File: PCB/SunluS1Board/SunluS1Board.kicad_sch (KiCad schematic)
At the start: 19 parts, among them M1 Fan, Q1 AO3400A, Q2 AO3400A, SW1 CS1213AGF260, SW2 CS1213AGF260, U1 STM32C011F4Px

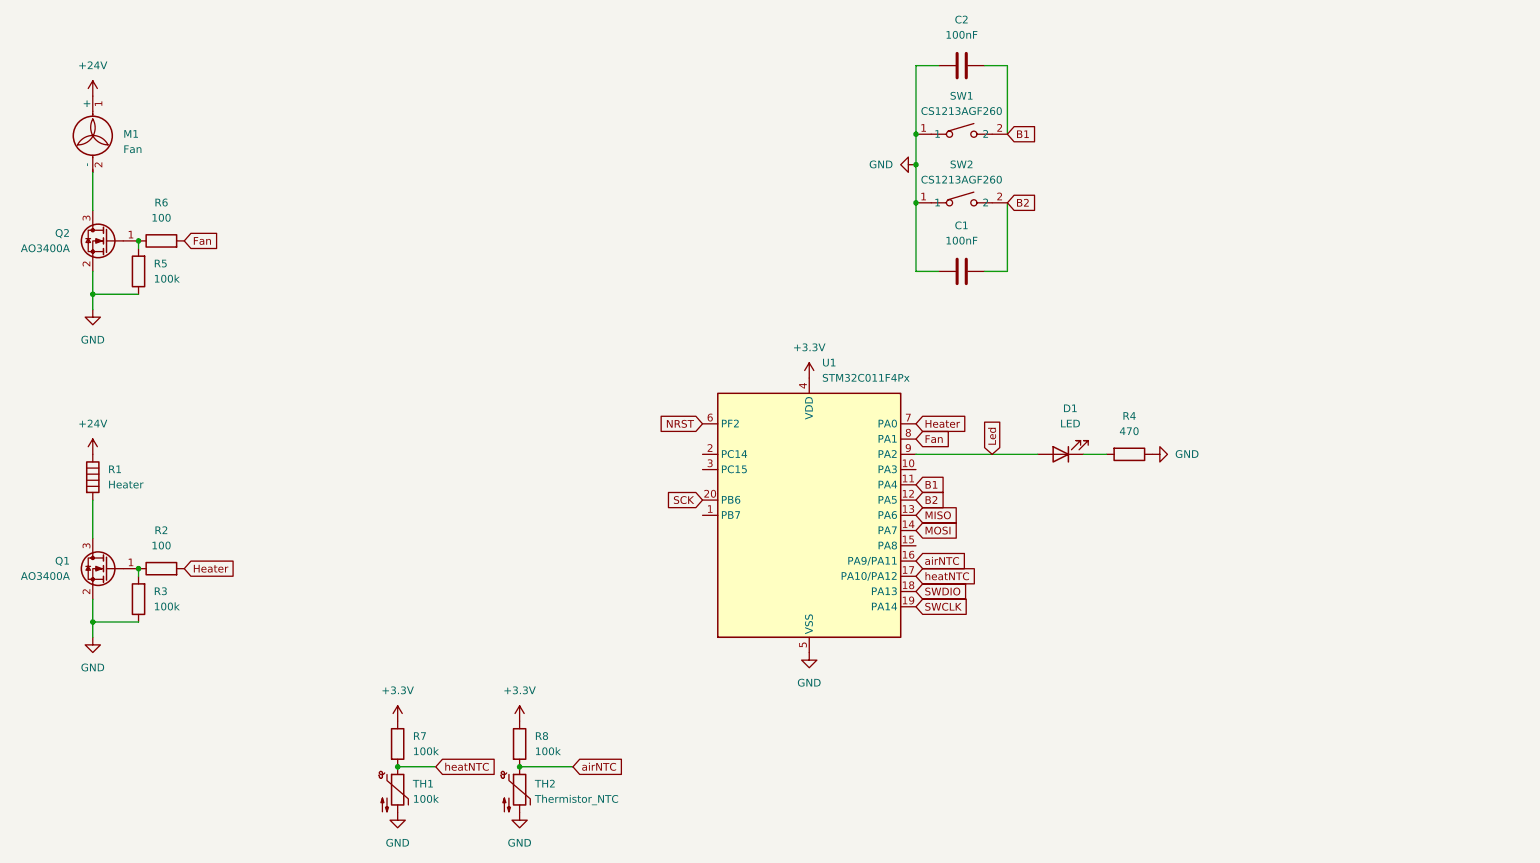
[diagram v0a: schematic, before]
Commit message: display
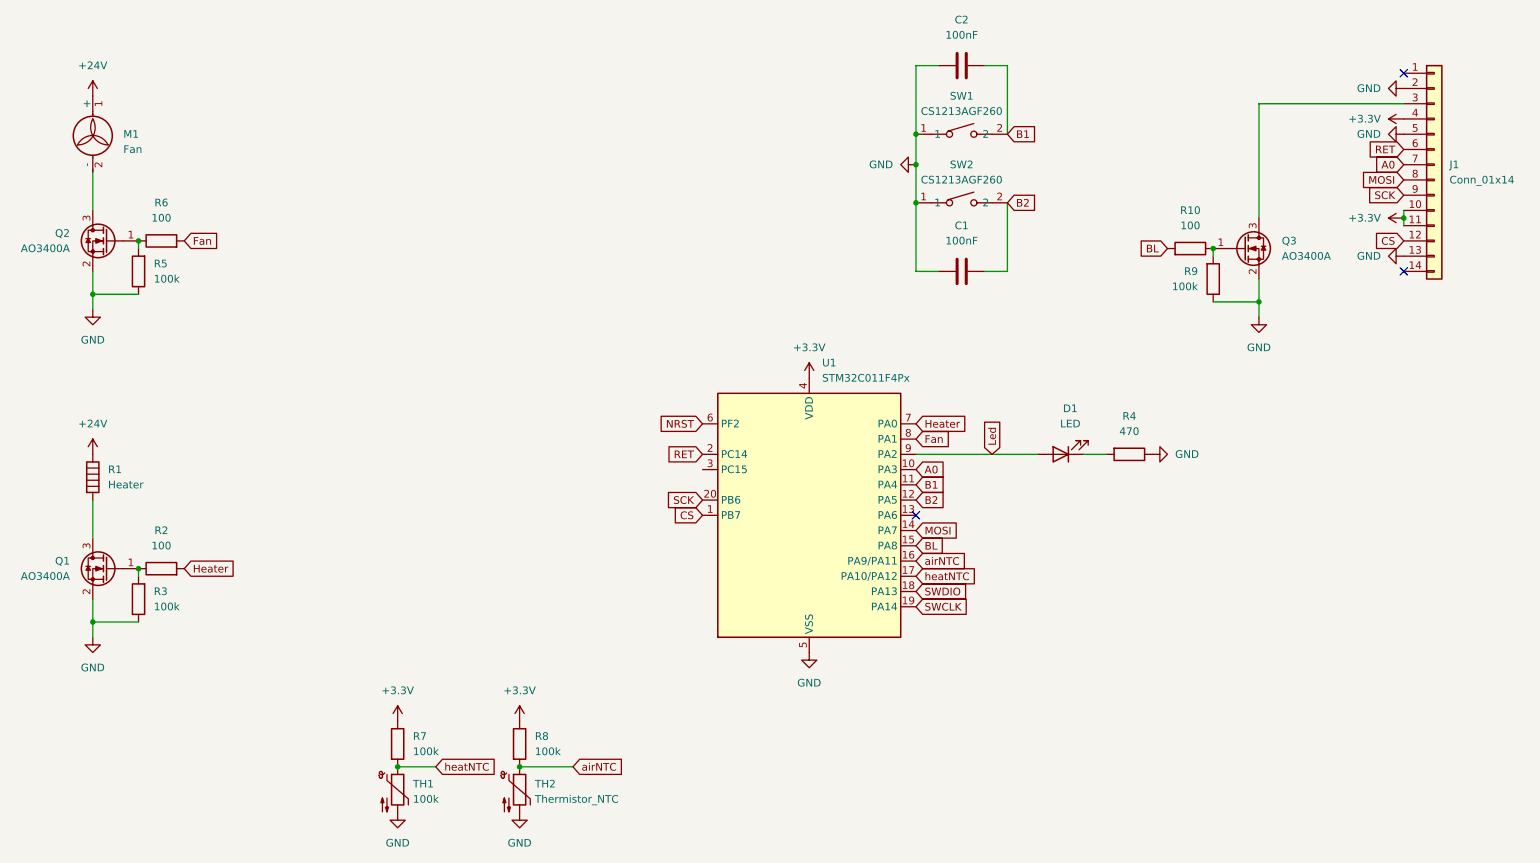
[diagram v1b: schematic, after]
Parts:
- added J1: Conn_01x14, symbol Connector_Generic:Conn_01x14
- added Q3: AO3400A, Package_TO_SOT_SMD:SOT-23, symbol Transistor_FET:AO3400A
- added R10: 100, symbol Device:R
- added R9: 100k, symbol Device:R
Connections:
- net +3.3V: now also J1.10 (Pin_10), J1.11 (Pin_11), J1.4 (Pin_4)
- net GND: now also J1.13 (Pin_13), J1.2 (Pin_2), J1.5 (Pin_5), Q3.2 (S), R9.1
- net MOSI: now also J1.8 (Pin_8)
- net SCK: now also J1.9 (Pin_9)
- net CS: now reaches U1.1 (PB7)
- net CS: now also J1.12 (Pin_12)
- net A0: now reaches U1.10 (PA3)
- net A0: now also J1.7 (Pin_7)
- net BL: now reaches U1.15 (PA8)
- net BL: now also R10.2
- net RET: now reaches U1.2 (PC14)
- net RET: now also J1.6 (Pin_6)
- net MISO: no longer names the net of U1.13 (PA6)
- new net: Q3.1 (G), R10.1, R9.2
- new net: J1.3 (Pin_3), Q3.3 (D)
- no-connect marks 0 -> 3
